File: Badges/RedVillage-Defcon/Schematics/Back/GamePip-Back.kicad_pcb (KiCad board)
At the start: 2 copper layers, 134.9 x 102.4 mm, 7 parts

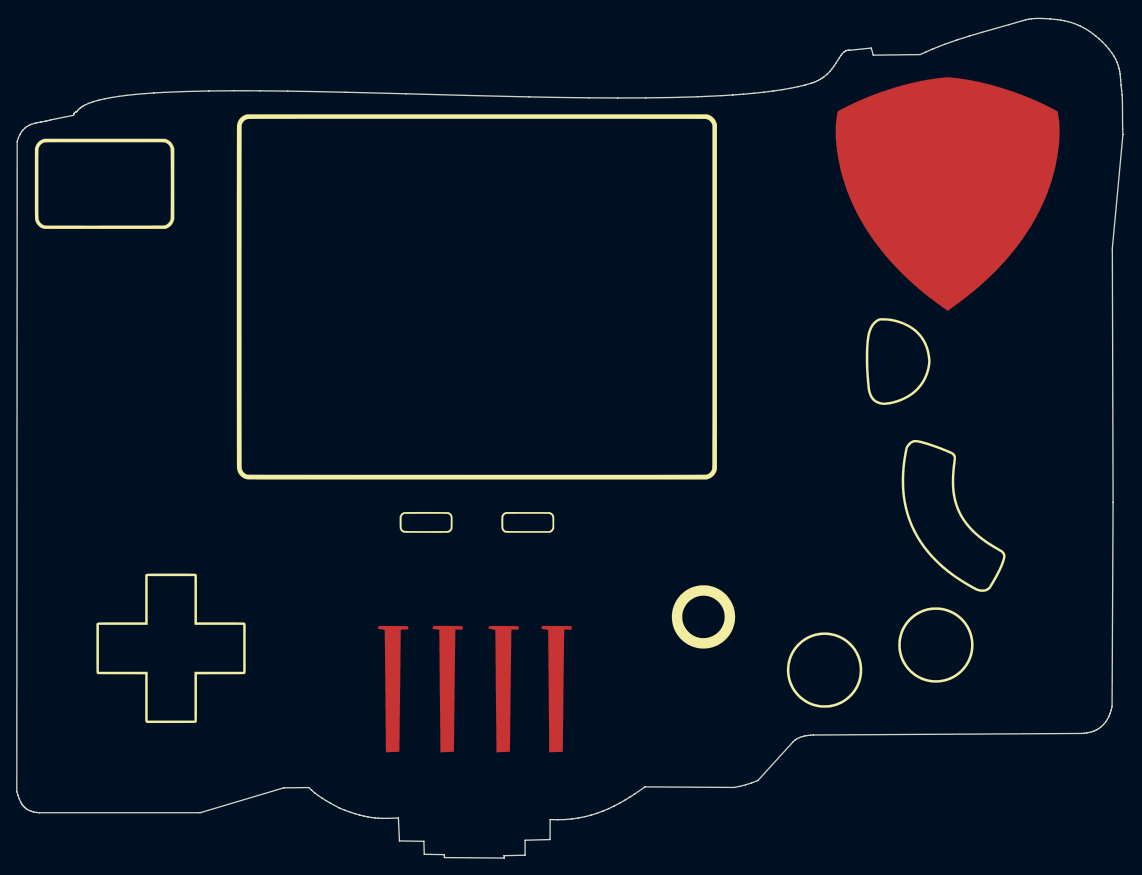
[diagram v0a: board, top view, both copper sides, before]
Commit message: Further updates
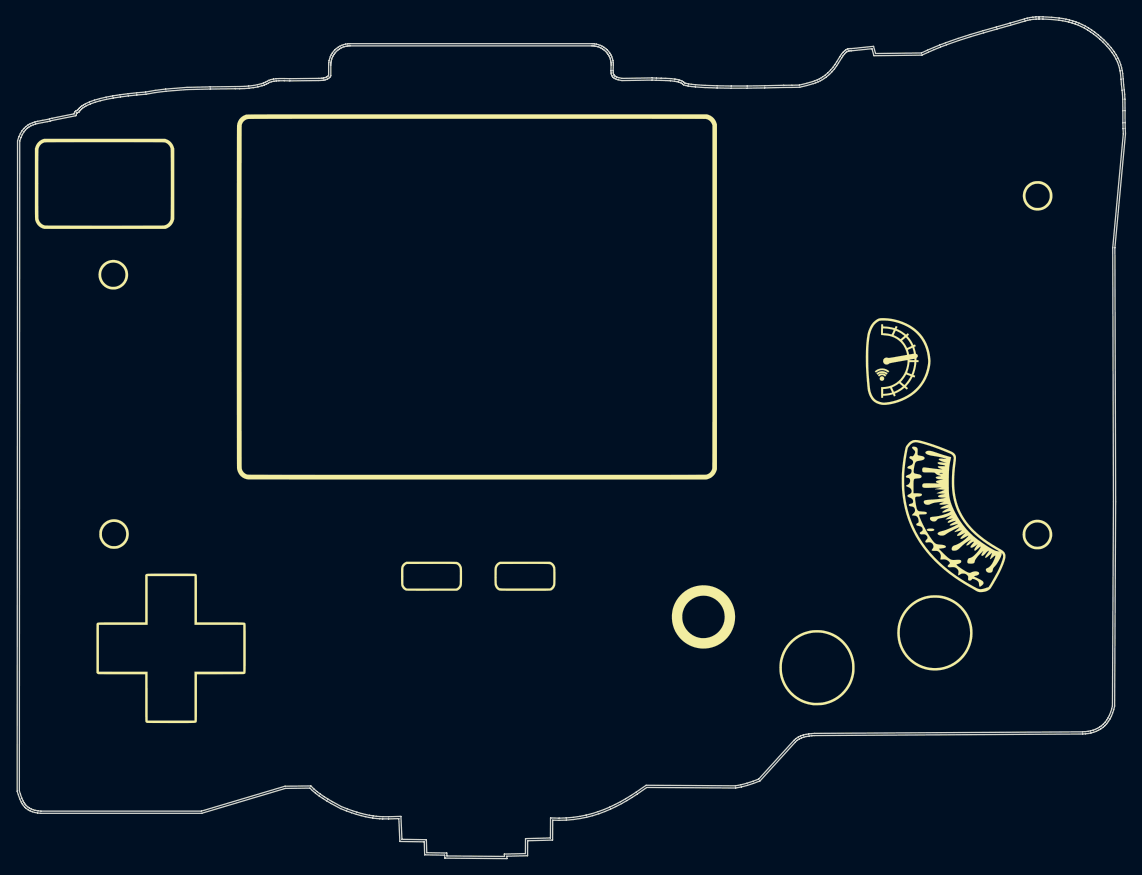
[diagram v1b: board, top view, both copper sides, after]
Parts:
- removed the G*** at (0.00, 0.00) (x7)
- added G*** (x7): LOGO, LOGO, F.Cu at (0.00, 0.00)
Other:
- board size 134.9 x 102.4 mm -> 135.2 x 102.7 mm
